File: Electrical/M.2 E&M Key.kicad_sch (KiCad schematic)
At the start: 28 parts, among them J1 Bus_M.2_Socket_M, J6 Bus_M.2_Socket_E

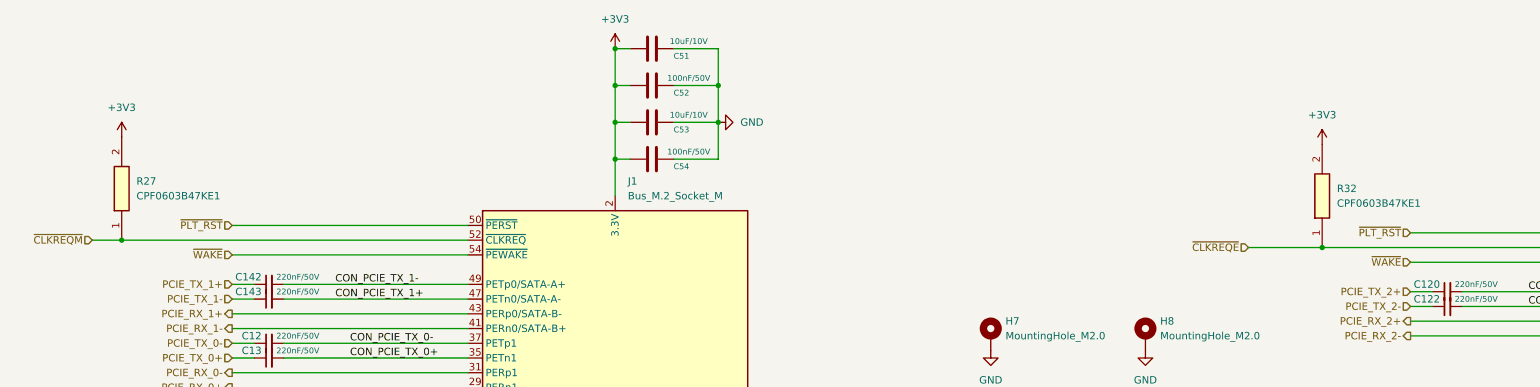
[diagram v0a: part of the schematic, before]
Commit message: Major Overhaul
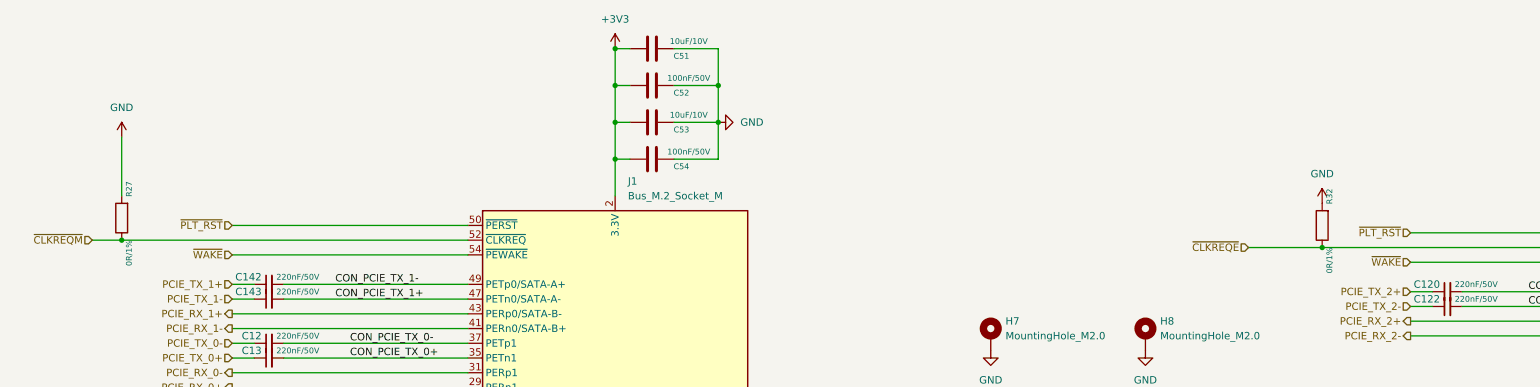
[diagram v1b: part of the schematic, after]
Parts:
- removed R27, R32: CPF0603B47KE1, 47k resis:RESC1608X55N, symbol 47k resis:CPF0603B47KE1
- added R27, R32: 0R/1%, A_HDJ_Library:R_0402_1005Metric, symbol Device:R
- H10, H7, H8, H9: footprint A_HDJ_Library:MountingHole_2.7mm_M2_Pad_TopOnly -> M.2:MountingHole_3mm_M2_Pad_TopOnly
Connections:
- net GND: now also R27.2, R32.2
- net ~{CLKREQE}: now also R32.1
- net ~{CLKREQM}: now also R27.1
